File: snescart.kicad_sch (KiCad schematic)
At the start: 5 parts, among them P1 CASSETTE, U2 27C512

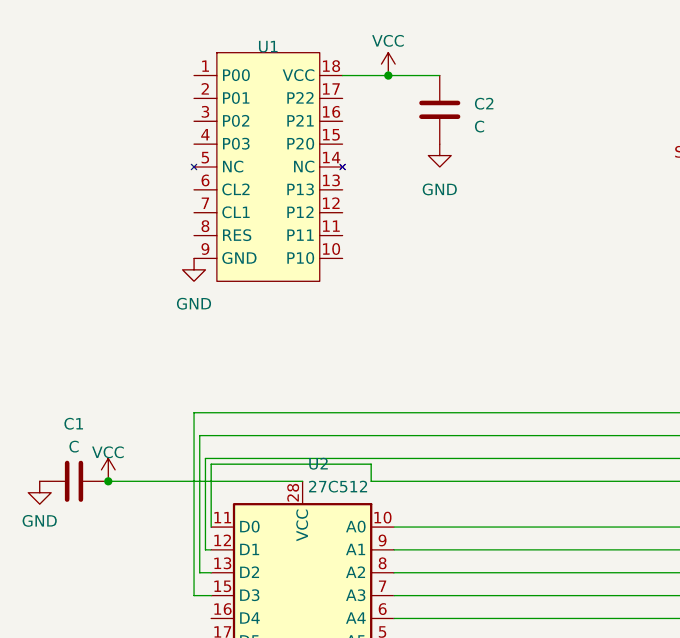
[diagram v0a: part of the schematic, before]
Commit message: fix cic
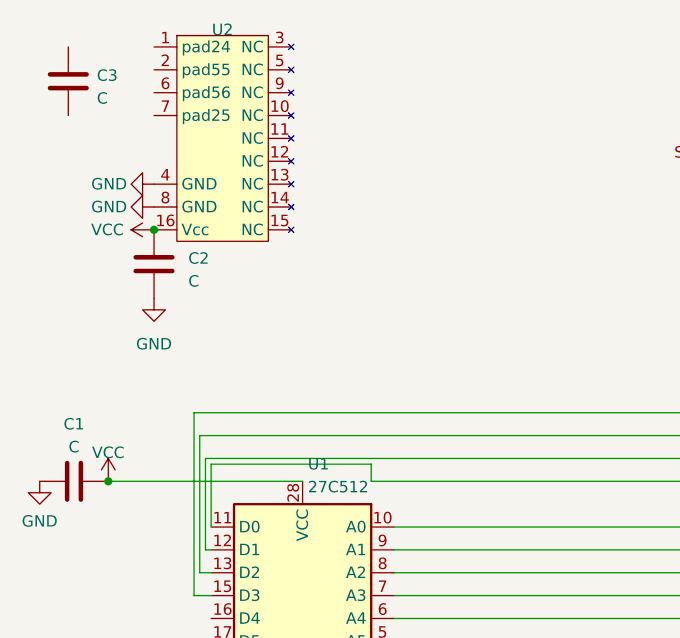
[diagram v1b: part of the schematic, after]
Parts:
- removed U1: ~, Package_DIP:DIP-18_W7.62mm, symbol SNES_Library:CIC
- added C3: C, Capacitor_THT:C_Disc_D4.3mm_W1.9mm_P5.00mm, symbol Device:C
- added U2: ~, Package_DIP:DIP-16_W7.62mm, symbol SNES_Library:CARTCIC
- renumbered U2 to U1
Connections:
- net GND: now also U2.4 (GND), U2.8 (GND)
- net VCC: now also U2.16 (Vcc)
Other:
- moved on the sheet: C2
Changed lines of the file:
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@@
 (kicad_sch (version 20230121) (generator eeschema)
   (paper "A4")
-  (junction (at 79.375 53.34) (diameter 0) (color 0 0 0 0)
+  (junction (at 53.34 70.485) (diameter 0) (color 0 0 0 0)
   )
   (junction (at 48.26 98.425) (diameter 0) (color 0 0 0 0)
@@
     (stroke (width 0) (type default))
   )
-  (wire (pts (xy 74.295 53.34) (xy 79.375 53.34))
-    (stroke (width 0) (type default))
-  )
   (wire (pts (xy 48.26 98.425) (xy 69.85 98.425))
     (stroke (width 0) (type default))
@@
     (stroke (width 0) (type default))
   )
-  (wire (pts (xy 79.375 53.34) (xy 85.09 53.34))
-    (stroke (width 0) (type default))
-  )
   (wire (pts (xy 80.01 121.285) (xy 113.03 121.285))
     (stroke (width 0) (type default))
@@
     (stroke (width 0) (type default))
   )
-  (symbol (lib_id "power:GND") (at 85.09 60.96 0) (unit 1)
-    (in_bom yes) (on_board yes) (dnp no) (fields_autoplaced)
-    (property "Reference" "#PWR06" (at 85.09 67.31 0)
-      (effects (font (size 1.27 1.27)) hide)
-    )
-    (property "Value" "GND" (at 85.09 66.04 0)
-      (effects (font (size 1.27 1.27)))
-    )
-    (property "Footprint" "" (at 85.09 60.96 0)
-      (effects (font (size 1.27 1.27)) hide)
-    )
-    (property "Datasheet" "" (at 85.09 60.96 0)
+  (symbol (lib_id "power:GND") (at 53.34 78.105 0) (unit 1)
+    (in_bom yes) (on_board yes) (dnp no) (fields_autoplaced)
+    (property "Reference" "#PWR06" (at 53.34 84.455 0)
+      (effects (font (size 1.27 1.27)) hide)
+    )
+    (property "Value" "GND" (at 53.34 83.185 0)
+      (effects (font (size 1.27 1.27)))
+    )
+    (property "Footprint" "" (at 53.34 78.105 0)
+      (effects (font (size 1.27 1.27)) hide)
+    )
+    (property "Datasheet" "" (at 53.34 78.105 0)
       (effects (font (size 1.27 1.27)) hide)
     )
@@
     )
   )
-  (symbol (lib_id "power:VCC") (at 79.375 53.34 0) (unit 1)
-    (in_bom yes) (on_board yes) (dnp no) (fields_autoplaced)
-    (property "Reference" "#PWR05" (at 79.375 57.15 0)
-      (effects (font (size 1.27 1.27)) hide)
-    )
-    (property "Value" "VCC" (at 79.375 49.53 0)
-      (effects (font (size 1.27 1.27)))
-    )
-    (property "Footprint" "" (at 79.375 53.34 0)
-      (effects (font (size 1.27 1.27)) hide)
-    )
-    (property "Datasheet" "" (at 79.375 53.34 0)
+  (symbol (lib_id "Device:C") (at 43.815 53.975 0) (unit 1)
+    (in_bom yes) (on_board yes) (dnp no) (fields_autoplaced)
+    (property "Reference" "C3" (at 46.99 53.34 0)
+      (effects (font (size 1.27 1.27)) (justify left))
+    )
+    (property "Value" "C" (at 46.99 55.88 0)
+      (effects (font (size 1.27 1.27)) (justify left))
+    )
+    (property "Footprint" "Capacitor_THT:C_Disc_D4.3mm_W1.9mm_P5.00mm" (at 44.7802 57.785 0)
+      (effects (font (size 1.27 1.27)) hide)
+    )
+    (property "Datasheet" "~" (at 43.815 53.975 0)
+      (effects (font (size 1.27 1.27)) hide)
+    )
+    (pin "1")
+    (pin "2")
+    (instances
+      (project "snescart"
+        (path "/066a4729-7396-4945-b543-8e17bff58a3f"
+          (reference "C3") (unit 1)
+        )
+      )
+    )
+  )
+  (symbol (lib_id "power:VCC") (at 53.34 70.485 90) (unit 1)
+    (in_bom yes) (on_board yes) (dnp no)
+    (property "Reference" "#PWR05" (at 57.15 70.485 0)
+      (effects (font (size 1.27 1.27)) hide)
+    )
+    (property "Value" "VCC" (at 46.355 70.485 90)
+      (effects (font (size 1.27 1.27)) (justify right))
+    )
+    (property "Footprint" "" (at 53.34 70.485 0)
+      (effects (font (size 1.27 1.27)) hide)
+    )
+    (property "Datasheet" "" (at 53.34 70.485 0)
       (effects (font (size 1.27 1.27)) hide)
     )
@@
     )
   )
-  (symbol (lib_id "Device:C") (at 85.09 57.15 0) (unit 1)
-    (in_bom yes) (on_board yes) (dnp no) (fields_autoplaced)
-    (property "Reference" "C2" (at 88.9 56.515 0)
+  (symbol (lib_id "Device:C") (at 53.34 74.295 0) (unit 1)
+    (in_bom yes) (on_board yes) (dnp no) (fields_autoplaced)
+    (property "Reference" "C2" (at 57.15 73.66 0)
       (effects (font (size 1.27 1.27)) (justify left))
     )
-    (property "Value" "C" (at 88.9 59.055 0)
+    (property "Value" "C" (at 57.15 76.2 0)
       (effects (font (size 1.27 1.27)) (justify left))
     )
-    (property "Footprint" "Capacitor_THT:C_Disc_D4.3mm_W1.9mm_P5.00mm" (at 86.0552 60.96 0)
-      (effects (font (size 1.27 1.27)) hide)
-    )
-    (property "Datasheet" "~" (at 85.09 57.15 0)
+    (property "Footprint" "Capacitor_THT:C_Disc_D4.3mm_W1.9mm_P5.00mm" (at 54.3052 78.105 0)
+      (effects (font (size 1.27 1.27)) hide)
+    )
+    (property "Datasheet" "~" (at 53.34 74.295 0)
       (effects (font (size 1.27 1.27)) hide)
     )
@@
   (symbol (lib_id "Memory_EPROM:27C512") (at 69.85 126.365 0) (mirror y) (unit 1)
     (in_bom yes) (on_board yes) (dnp no) (fields_autoplaced)
-    (property "Reference" "U2" (at 70.4341 96.52 0)
+    (property "Reference" "U1" (at 70.4341 96.52 0)
       (effects (font (size 1.27 1.27)) (justify right))
     )
@@
       (project "snescart"
         (path "/066a4729-7396-4945-b543-8e17bff58a3f"
-          (reference "U2") (unit 1)
+          (reference "U1") (unit 1)
         )
       )
@@
     )
   )
+  (symbol (lib_id "power:GND") (at 53.34 65.405 270) (unit 1)
+    (in_bom yes) (on_board yes) (dnp no)
+    (property "Reference" "#PWR09" (at 46.99 65.405 0)
+      (effects (font (size 1.27 1.27)) hide)
+    )
+    (property "Value" "GND" (at 46.355 65.405 90)
+      (effects (font (size 1.27 1.27)) (justify left))
+    )
+    (property "Footprint" "" (at 53.34 65.405 0)
+      (effects (font (size 1.27 1.27)) hide)
+    )
+    (property "Datasheet" "" (at 53.34 65.405 0)
+      (effects (font (size 1.27 1.27)) hide)
+    )
+    (pin "1")
+    (instances
+      (project "snescart"
+        (path "/066a4729-7396-4945-b543-8e17bff58a3f"
+          (reference "#PWR09") (unit 1)
+        )
+      )
+    )
+  )
   (symbol (lib_id "power:GND") (at 138.43 133.985 90) (unit 1)
     (in_bom yes) (on_board yes) (dnp no) (fields_autoplaced)
@@
         (path "/066a4729-7396-4945-b543-8e17bff58a3f"
           (reference "#PWR08") (unit 1)
-        )
-      )
-    )
-  )
-  (symbol (lib_id "SNES_Library:CIC") (at 66.675 62.23 0) (unit 1)
-    (in_bom yes) (on_board yes) (dnp no) (fields_autoplaced)
-    (property "Reference" "U1" (at 66.04 50.165 0)
-      (effects (font (size 1.27 1.27)))
-    )
-    (property "Value" "~" (at 61.595 48.26 0)
-      (effects (font (size 1.27 1.27)))
-    )
-    (property "Footprint" "Package_DIP:DIP-18_W7.62mm" (at 61.595 48.26 0)
-      (effects (font (size 1.27 1.27)) hide)
-    )
-    (property "Datasheet" "" (at 61.595 48.26 0)
-      (effects (font (size 1.27 1.27)) hide)
-    )
-    (pin "1")
-    (pin "10")
-    (pin "11")
-    (pin "12")
-    (pin "13")
-    (pin "14")
-    (pin "15")
-    (pin "16")
-    (pin "17")
-    (pin "18")
-    (pin "2")
-    (pin "3")
-    (pin "4")
-    (pin "5")
-    (pin "6")
-    (pin "7")
-    (pin "8")
-    (pin "9")
-    (instances
-      (project "snescart"
-        (path "/066a4729-7396-4945-b543-8e17bff58a3f"
-          (reference "U1") (unit 1)
         )
       )
@@
     )
   )
-  (symbol (lib_id "power:GND") (at 57.785 73.66 0) (unit 1)
-    (in_bom yes) (on_board yes) (dnp no) (fields_autoplaced)
-    (property "Reference" "#PWR04" (at 57.785 80.01 0)
-      (effects (font (size 1.27 1.27)) hide)
-    )
-    (property "Value" "GND" (at 57.785 78.74 0)
-      (effects (font (size 1.27 1.27)))
-    )
-    (property "Footprint" "" (at 57.785 73.66 0)
-      (effects (font (size 1.27 1.27)) hide)
-    )
-    (property "Datasheet" "" (at 57.785 73.66 0)
+  (symbol (lib_id "power:GND") (at 53.34 67.945 270) (unit 1)
+    (in_bom yes) (on_board yes) (dnp no)
+    (property "Reference" "#PWR04" (at 46.99 67.945 0)
+      (effects (font (size 1.27 1.27)) hide)
+    )
+    (property "Value" "GND" (at 46.355 67.945 90)
+      (effects (font (size 1.27 1.27)) (justify left))
+    )
+    (property "Footprint" "" (at 53.34 67.945 0)
+      (effects (font (size 1.27 1.27)) hide)
+    )
+    (property "Datasheet" "" (at 53.34 67.945 0)
       (effects (font (size 1.27 1.27)) hide)
     )
@@
         )
       )
+    )
+  )
+  (symbol (lib_id "SNES_Library:CARTCIC") (at 60.96 59.055 0) (unit 1)
+    (in_bom yes) (on_board yes) (dnp no) (fields_autoplaced)
+    (property "Reference" "U2" (at 60.96 48.26 0)
+      (effects (font (size 1.27 1.27)))
+    )
+    (property "Value" "~" (at 53.34 50.165 0)
+      (effects (font (size 1.27 1.27)))
+    )
+    (property "Footprint" "Package_DIP:DIP-16_W7.62mm" (at 53.34 50.165 0)
+      (effects (font (size 1.27 1.27)) hide)
+    )
+    (property "Datasheet" "" (at 53.34 50.165 0)
+      (effects (font (size 1.27 1.27)) hide)
+    )
+    (pin "1")
+    (pin "10")
+    (pin "11")
+    (pin "12")
+    (pin "13")
+    (pin "14")
+    (pin "15")
+    (pin "16")
+    (pin "2")
+    (pin "3")
+    (pin "4")
+    (pin "5")
+    (pin "6")
+    (pin "7")
+    (pin "8")
+    (pin "9")
+    (instances
+      (project "snescart"
+        (path "/066a4729-7396-4945-b543-8e17bff58a3f"
+          (reference "U2") (unit 1)
+        )
+      )

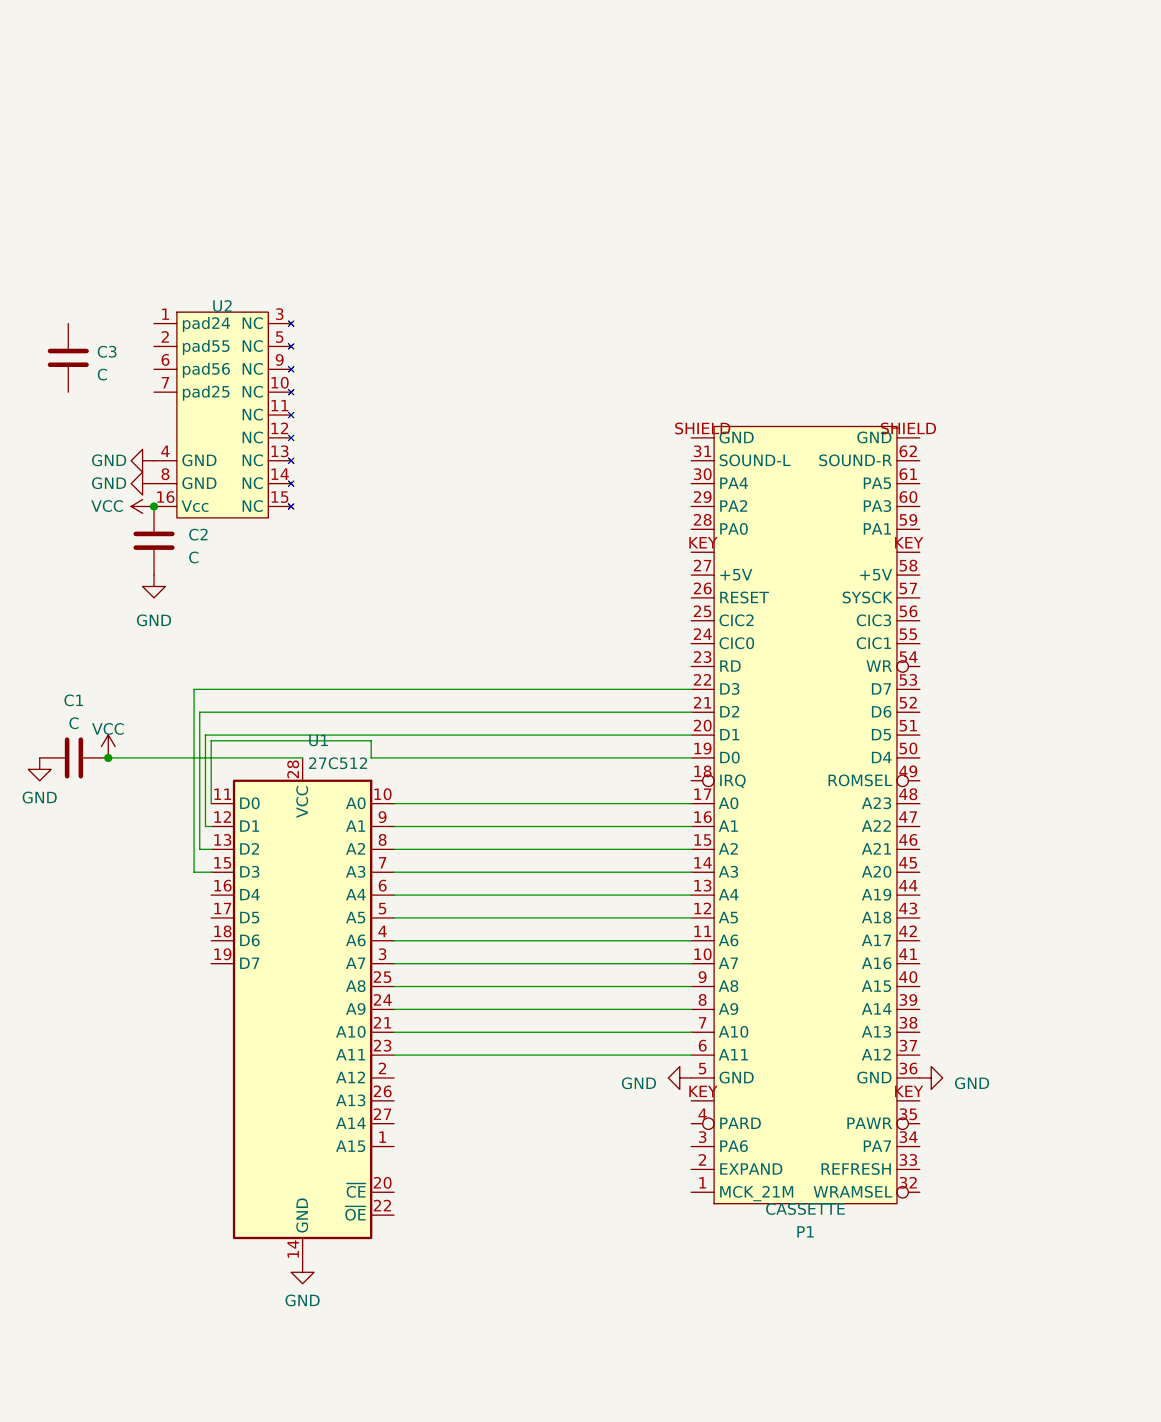
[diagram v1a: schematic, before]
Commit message: feet
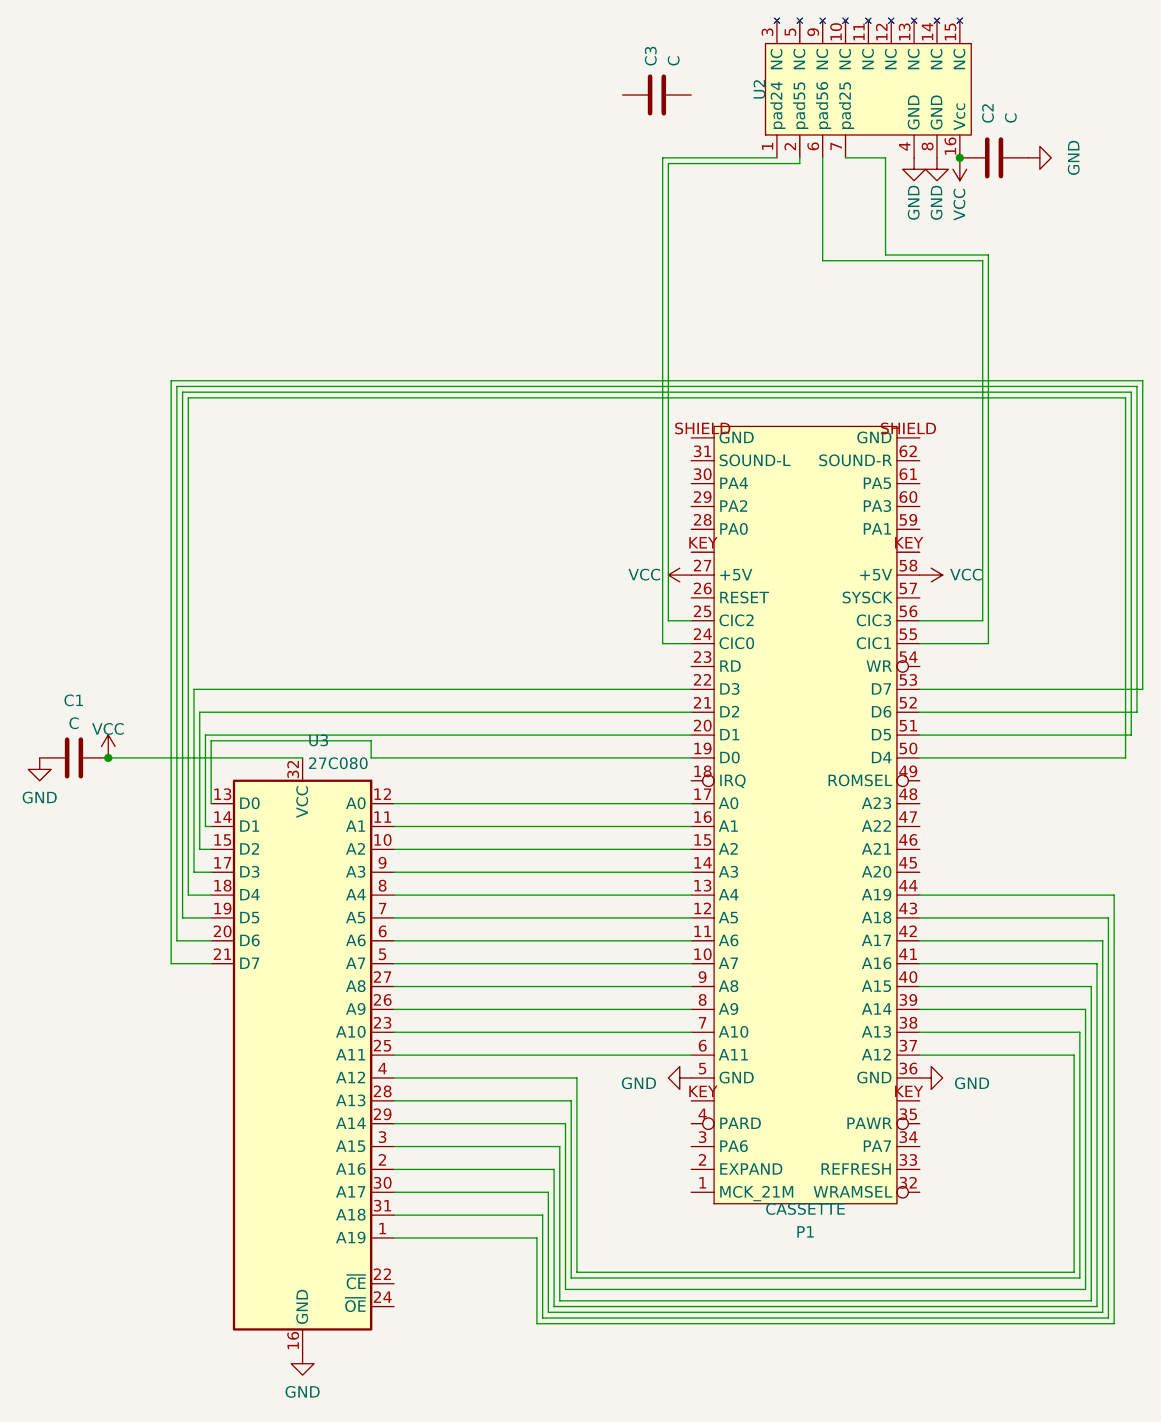
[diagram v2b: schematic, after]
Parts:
- removed U1: 27C512, Package_DIP:DIP-28_W15.24mm, symbol Memory_EPROM:27C512
- added U3: 27C080, symbol Memory_EPROM:27C080
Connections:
- net GND: now also U3.16 (GND)
- net VCC: now also P1.27 (+5V), P1.58 (+5V), U3.32 (VCC)
- net at P1.17 (A0): now also U3.12 (A0)
- net at P1.19 (D0): now also U3.13 (D0)
- net at P1.20 (D1): now also U3.14 (D1)
- net at P1.21 (D2): now also U3.15 (D2)
- net at P1.22 (D3): now also U3.17 (D3)
- net at P1.7 (A10): now also U3.23 (A10)
- net at P1.6 (A11): now also U3.25 (A11)
- net at P1.8 (A9): now also U3.26 (A9)
- net at P1.9 (A8): now also U3.27 (A8)
- net at P1.10 (A7): now also U3.5 (A7)
- net at P1.11 (A6): now also U3.6 (A6)
- net at P1.12 (A5): now also U3.7 (A5)
- net at P1.13 (A4): now also U3.8 (A4)
- net at P1.14 (A3): now also U3.9 (A3)
- net at P1.15 (A2): now also U3.10 (A2)
- net at P1.16 (A1): now also U3.11 (A1)
- net at P1.24 (CIC0): now also U2.1 (pad24)
- net at P1.25 (CIC2): now also U2.2 (pad55)
- net at P1.37 (A12): now also U3.4 (A12)
- net at P1.38 (A13): now also U3.28 (A13)
- net at P1.39 (A14): now also U3.29 (A14)
- net at P1.40 (A15): now also U3.3 (A15)
- net at P1.41 (A16): now also U3.2 (A16)
- net at P1.42 (A17): now also U3.30 (A17)
- net at P1.43 (A18): now also U3.31 (A18)
- net at P1.44 (A19): now also U3.1 (A19)
- net at P1.50 (D4): now also U3.18 (D4)
- net at P1.51 (D5): now also U3.19 (D5)
- net at P1.52 (D6): now also U3.20 (D6)
- net at P1.53 (D7): now also U3.21 (D7)
- net at P1.55 (CIC1): now also U2.7 (pad25)
- net at P1.56 (CIC3): now also U2.6 (pad56)
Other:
- moved on the sheet: C2, C3, U2
